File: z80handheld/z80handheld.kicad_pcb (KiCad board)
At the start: 2 copper layers, 105.2 x 148.2 mm, 139 parts, among them IC1 DS12885+, J1 Power, J2 Esp32 C3 Supermini Right, J3 SPI Screen, J4 Esp32 C3 Supermini Left, J5 Conn_01x40, SW1 SW_Push_45deg, SW10 SW_Push_45deg, SW11 SW_Push_45deg, SW12 SW_Push_45deg, SW13 SW_Push_45deg, SW14 SW_Push_45deg, SW15 SW_Push_45deg, SW16 SW_Push_45deg, SW17 SW_Push_45deg, SW18 SW_Push_45deg, SW19 SW_Push_45deg, SW2 SW_Push_45deg, SW20 SW_Push_45deg, SW21 SW_Push_45deg, SW22 SW_Push_45deg, SW23 SW_Push_45deg, SW24 SW_Push_45deg, SW25 SW_Push_45deg, SW26 SW_Push_45deg, SW27 SW_Push_45deg, SW28 SW_Push_45deg, SW29 SW_Push_45deg, SW3 SW_Push_45deg, SW30 SW_Push_45deg, SW31 SW_Push_45deg, SW32 SW_Push_45deg, SW33 SW_Push_45deg, SW34 SW_Push_45deg, SW35 SW_Push_45deg, SW36 SW_Push_45deg, SW37 SW_Push_45deg, SW38 SW_Push_45deg, SW39 SW_Push_45deg, SW4 SW_Push_45deg, SW40 SW_Push_45deg, SW41 SW_Push_45deg, SW42 SW_Push_45deg, SW43 SW_Push_45deg, SW44 SW_Push_45deg, SW45 SW_Push_45deg, SW46 SW_Push_45deg, SW47 SW_Push_45deg, SW48 SW_Push_45deg, SW49 SW_Push_45deg, SW5 SW_Push_45deg, SW50 SW_Push_45deg, SW51 SW_Push_45deg, SW52 SW_Push_45deg, SW53 SW_Push_45deg, SW54 SW_Push_45deg, SW55 SW_Push_45deg, SW56 SW_Push_45deg, SW57 SW_Push_45deg, SW58 SW_Push_45deg, SW59 SW_Push_45deg, SW6 SW_Push_45deg, SW60 SW_Push_45deg, SW61 SW_Push_45deg, SW62 SW_Push_45deg, SW63 SW_Push_45deg, SW64 SW_Push_45deg, SW65 SW_Push, SW7 SW_Push_45deg, SW8 SW_Push_45deg, SW9 SW_Push_45deg, U1 74HC04, U10 Z84C00xxP, U11 74LS573 IO1, U12 HDSP-7501, U13 74LS573, U14 HDSP-7501, U15 74LS573, U16 16550 IO2, U17 16550 IO3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

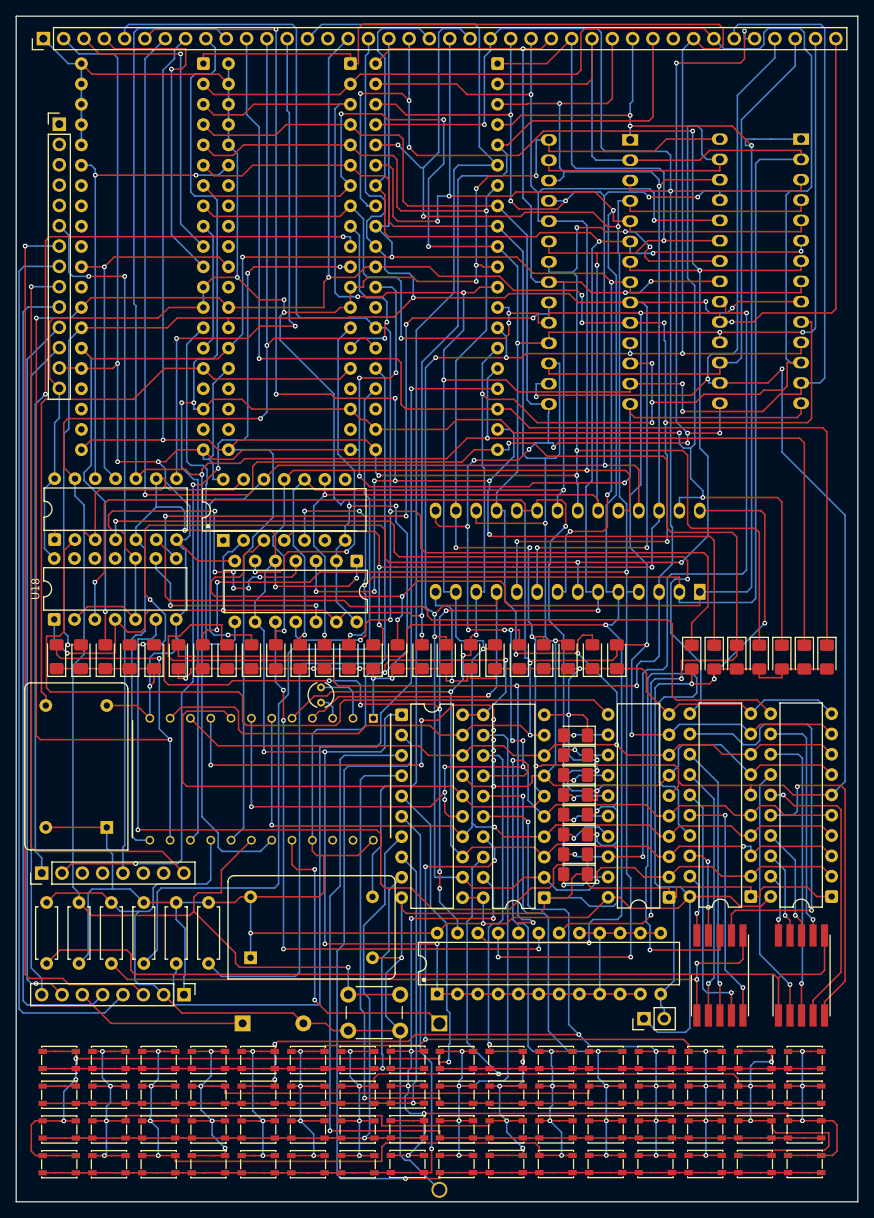
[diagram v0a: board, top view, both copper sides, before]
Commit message: Add files via upload
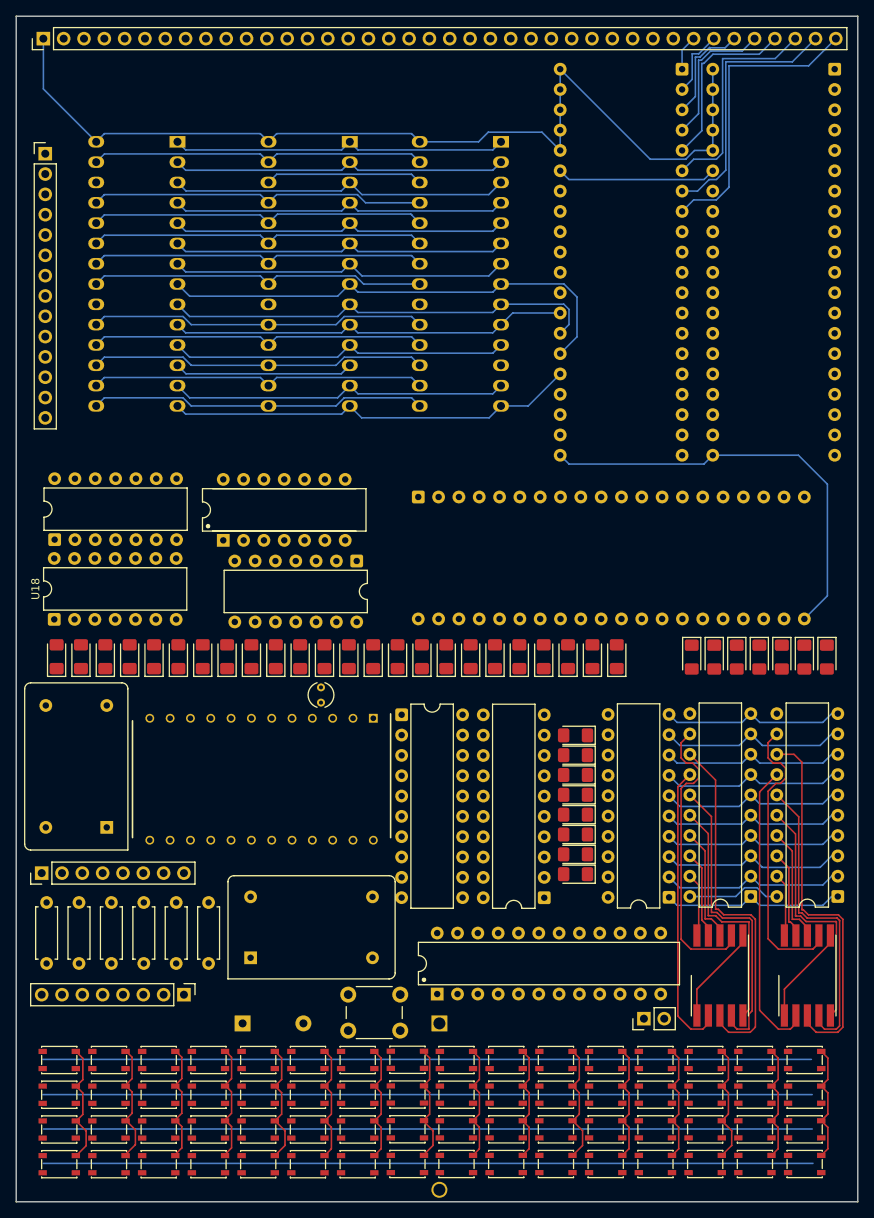
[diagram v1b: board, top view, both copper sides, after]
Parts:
- moved U8 61.5 mm to (265.6, 83.0), turned to 180 degrees
- moved U16 60.5 mm to (307.3, 73.9)
- moved U17 59.9 mm to (288.2, 73.9)
- moved U9 56.6 mm to (225.2, 83.0)
- moved U7 56.4 mm to (246.7, 83.0)
- moved U10 55.1 mm to (255.3, 127.4), turned to -90 degrees
- moved J3 4.09 mm to (208.6, 84.5)
- moved U15 0.77 mm to (307.7, 177.3)
- moved U14 0.73 mm to (303.9, 187.2)
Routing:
- net GND: track 685.7 -> 97.3 mm, vias 22 -> 0
- net 5V: track 616.3 -> 133.1 mm, vias 16 -> 0
- net (no net): track 0.00 -> 384.7 mm
- net /D4: track 380.3 -> 87.6 mm, vias 8 -> 0
- net /D1: track 326.7 -> 54.1 mm, vias 8 -> 0
- net /D0: track 342.2 -> 70.1 mm, vias 8 -> 0
- net /D2: track 341.0 -> 78.6 mm, vias 8 -> 0
- net /A0: track 310.9 -> 50.1 mm, vias 10 -> 0
- net IO1: track 255.0 -> 0.00 mm, vias 7 -> 0
- net /D3: track 333.2 -> 82.7 mm, vias 19 -> 0
- net !WR: track 290.8 -> 42.1 mm, vias 4 -> 0
- net !INT: track 244.4 -> 0.00 mm, vias 2 -> 0
- net /D5: track 326.4 -> 93.2 mm, vias 11 -> 0
- net /A7: track 264.7 -> 42.6 mm, vias 5 -> 0
- net /A6: track 263.8 -> 42.1 mm, vias 8 -> 0
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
